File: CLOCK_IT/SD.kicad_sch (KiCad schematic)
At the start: 3 parts

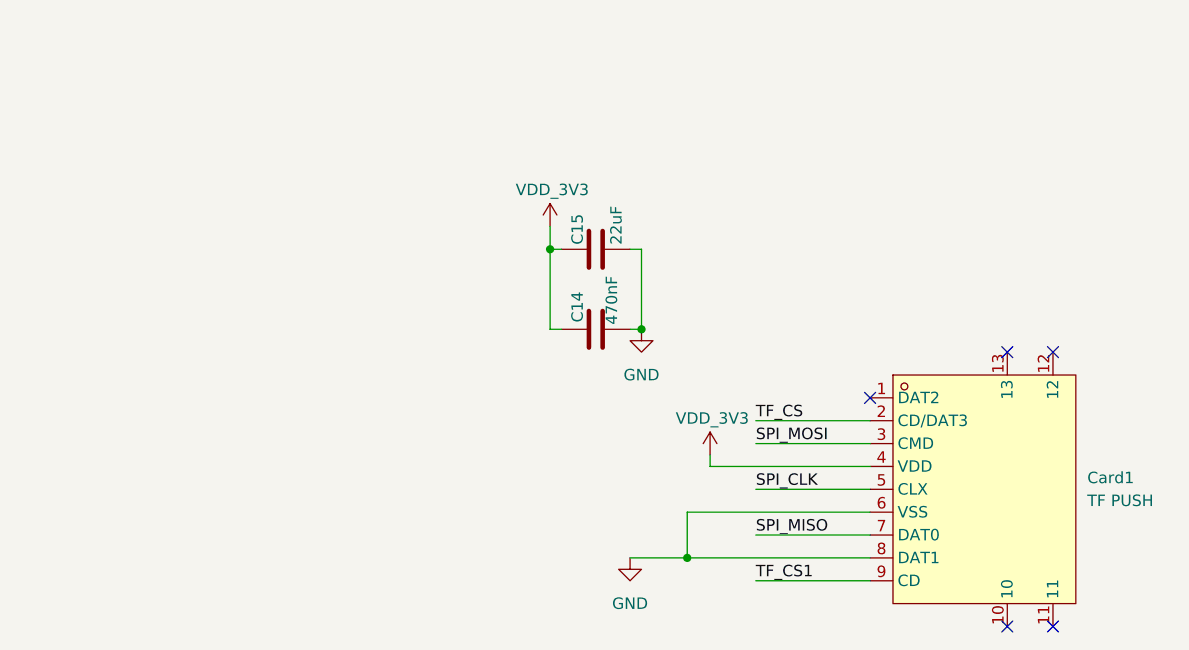
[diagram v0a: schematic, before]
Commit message: :memo: Sfinished -TF-
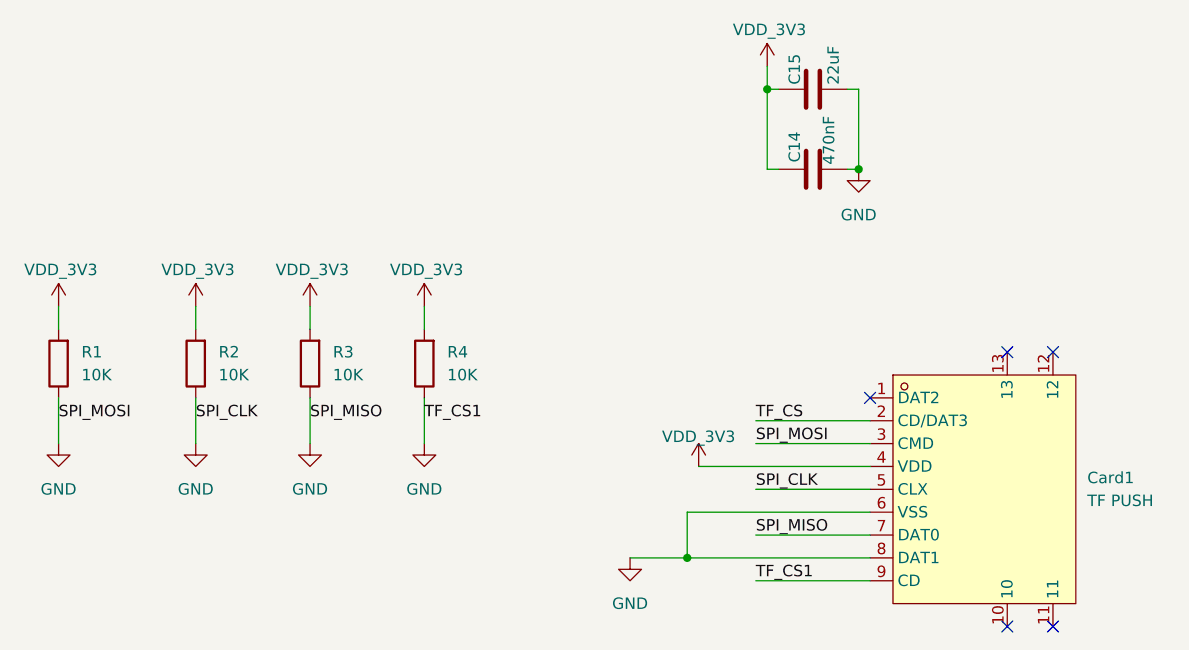
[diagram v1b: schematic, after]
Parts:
- added R1, R2, R3, R4: 10K, symbol Device:R
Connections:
- net SPI_CLK is gone; now on net GND: Card1.5 (CLX)
- net SPI_MISO is gone; now on net GND: Card1.7 (DAT0)
- net SPI_MOSI is gone; now on net GND: Card1.3 (CMD)
- net TF_CS1 is gone; now on net GND: Card1.9 (CD)
- net GND: now also R1.1, R2.1, R3.1, R4.1
- net VDD_3V3: now also R1.2, R2.2, R3.2, R4.2
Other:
- moved on the sheet: C14, C15
